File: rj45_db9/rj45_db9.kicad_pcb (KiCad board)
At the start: 2 copper layers, 30 x 32 mm, 2 parts, among them J1 RJ45_LED, J2 DB9_Female

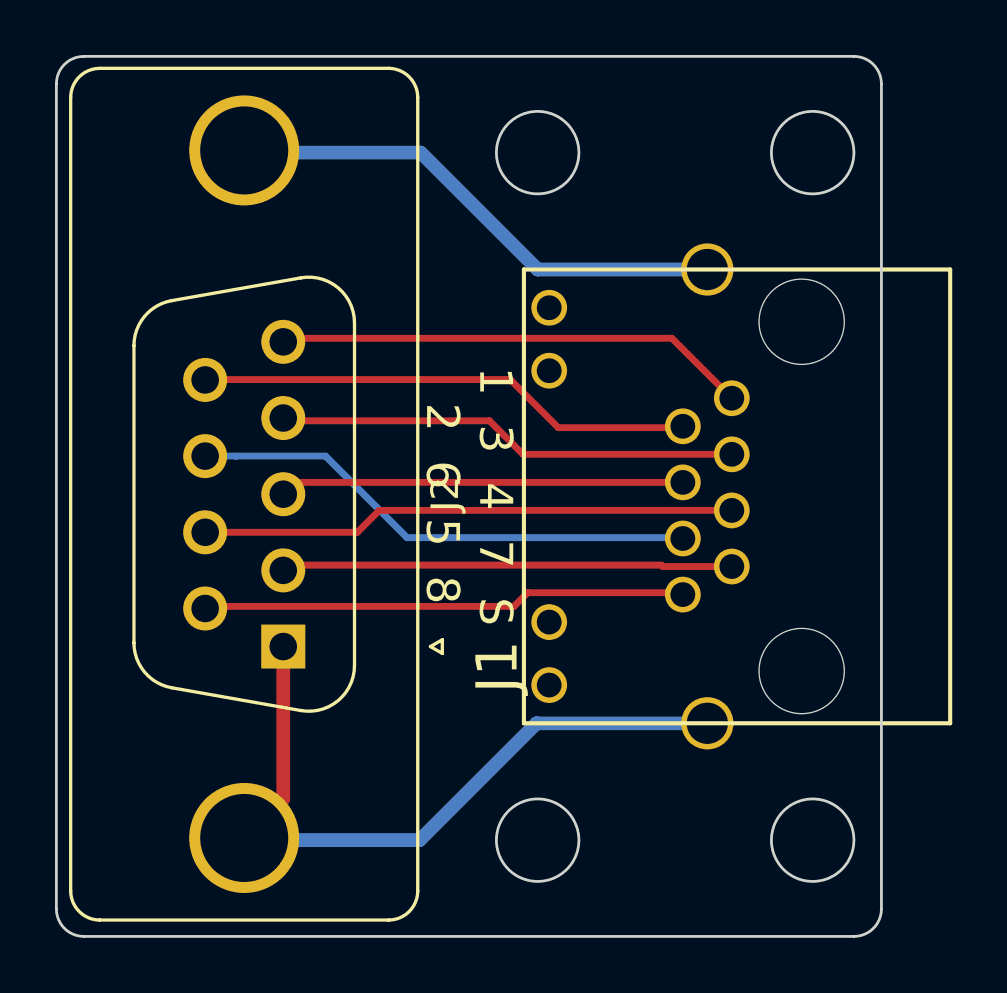
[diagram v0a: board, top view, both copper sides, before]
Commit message: hw
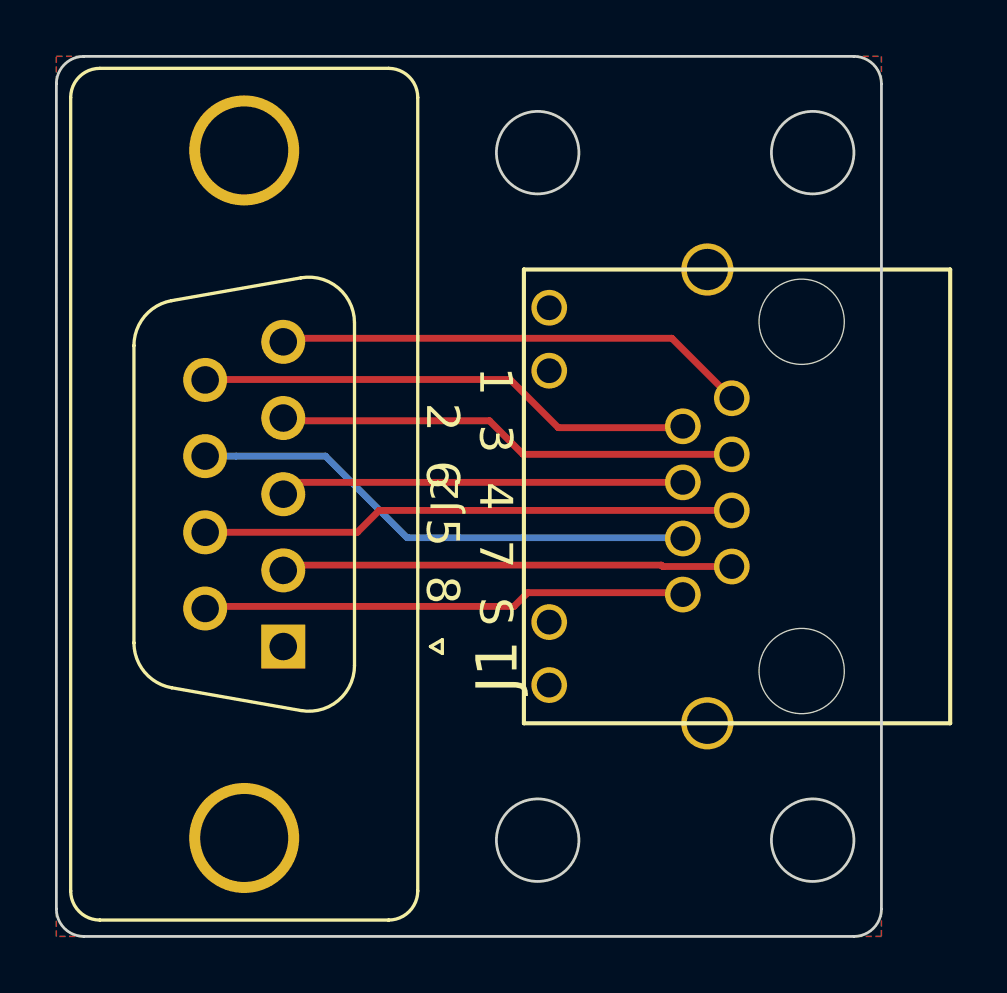
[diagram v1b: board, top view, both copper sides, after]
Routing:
- net Net-(J1-Pad13): track 44.6 -> 0.00 mm
- added copper zone on B.Cu, net Net-(J1-Pad13)
- added copper zone on F.Cu, net Net-(J1-Pad13)
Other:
- net class Default: via_dia 0.8 -> 0.6; via_drill 0.4 -> 0.3
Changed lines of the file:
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@@
     (thickness 1.6)
     (drawings 13)
-    (tracks 39)
+    (tracks 31)
     (zones 0)
     (modules 2)
@@
     (last_trace_width 0.25)
     (trace_clearance 0.2)
-    (zone_clearance 0.508)
+    (zone_clearance 0.2)
     (zone_45_only no)
     (trace_min 0.2)
-    (via_size 0.8)
-    (via_drill 0.4)
+    (via_size 0.6)
+    (via_drill 0.3)
     (via_min_size 0.4)
     (via_min_drill 0.3)
@@
     (clearance 0.2)
     (trace_width 0.25)
-    (via_dia 0.8)
-    (via_drill 0.4)
+    (via_dia 0.6)
+    (via_drill 0.3)
     (uvia_dia 0.3)
     (uvia_drill 0.1)
     (add_net "Net-(J1-Pad1)")
-    (add_net "Net-(J1-Pad10)")
-    (add_net "Net-(J1-Pad11)")
-    (add_net "Net-(J1-Pad12)")
     (add_net "Net-(J1-Pad13)")
     (add_net "Net-(J1-Pad2)")
@@
     (add_net "Net-(J1-Pad7)")
     (add_net "Net-(J1-Pad8)")
-    (add_net "Net-(J1-Pad9)")
   )
   (module stmbl:DSUB-9_Female_Vertical_Pitch2.77x2.84mm_MountingHoles (layer F.Cu)
@@
   (gr_line (start 143.5 116) (end 171.5 116) (layer Edge.Cuts) (width 0.1))
   (gr_line (start 142.5 85) (end 142.5 115) (layer Edge.Cuts) (width 0.1))
-  (segment (start 160 91.75) (end 166.17 91.75) (width 0.5) (layer B.Cu) (net 1))
-  (segment (start 155.75 87.5) (end 160 91.75) (width 0.5) (layer B.Cu) (net 1))
-  (segment (start 149.42 87.5) (end 155.75 87.5) (width 0.5) (layer B.Cu) (net 1))
-  (segment (start 155.71 112.5) (end 159.96 108.25) (width 0.5) (layer B.Cu) (net 1))
-  (segment (start 159.96 108.25) (end 166.17 108.25) (width 0.5) (layer B.Cu) (net 1))
-  (segment (start 149.42 112.5) (end 155.71 112.5) (width 0.5) (layer B.Cu) (net 1))
-  (segment (start 150.75 111) (end 150.75 105.46) (width 0.5) (layer F.Cu) (net 1))
-  (segment (start 149.33 112.42) (end 150.75 111) (width 0.5) (layer F.Cu) (net 1))
   (segment (start 164.88 94.25) (end 167.06 96.43) (width 0.25) (layer F.Cu) (net 2))
   (segment (start 150.75 94.38) (end 150.88 94.25) (width 0.25) (layer F.Cu) (net 2))
@@
   (segment (start 159.14 104) (end 159.64 103.5) (width 0.25) (layer F.Cu) (net 9))
   (segment (start 159.64 103.5) (end 165.21 103.5) (width 0.25) (layer F.Cu) (net 9))
+  (zone (net 1) (net_name "Net-(J1-Pad13)") (layer F.Cu) (hatch edge 0.508)
+    (connect_pads (clearance 0.2))
+    (min_thickness 0.2)
+    (fill yes (arc_segments 32) (thermal_gap 0.2) (thermal_bridge_width 0.25))
+    (polygon
+      (pts
+        (xy 142.5 84) (xy 172.5 84) (xy 172.5 116) (xy 142.5 116)
+      )
+    )
+  )
+  (zone (net 1) (net_name "Net-(J1-Pad13)") (layer B.Cu) (hatch edge 0.508)
+    (connect_pads (clearance 0.2))
+    (min_thickness 0.2)
+    (fill yes (arc_segments 32) (thermal_gap 0.2) (thermal_bridge_width 0.25))
+    (polygon
+      (pts
+        (xy 142.5 84) (xy 172.5 84) (xy 172.5 116) (xy 142.5 116)
+      )
+    )
+  )
+  (zone (net 0) (net_name "") (layers F&B.Cu) (hatch edge 0.508)
+    (connect_pads (clearance 0.2))
+    (min_thickness 0.2)
+    (keepout (tracks not_allowed) (vias not_allowed) (copperpour not_allowed))
+    (fill (arc_segments 32) (thermal_gap 0.2) (thermal_bridge_width 0.25))
+    (polygon
+      (pts
+        (xy 160 108.75) (xy 162 108.75) (xy 163.75 110.5) (xy 163.75 116) (xy 156.25 116)
+        (xy 156.25 110.5) (xy 158 108.75)
+      )
+    )
+  )
+  (zone (net 0) (net_name "") (layers F&B.Cu) (hatch edge 0.508)
+    (connect_pads (clearance 0.2))
+    (min_thickness 0.2)
+    (keepout (tracks not_allowed) (vias not_allowed) (copperpour not_allowed))
+    (fill (arc_segments 32) (thermal_gap 0.2) (thermal_bridge_width 0.25))
+    (polygon
+      (pts
+        (xy 169.978671 108.75) (xy 172.478671 108.75) (xy 173.728671 110) (xy 173.728671 116) (xy 166.228671 116)
+        (xy 166.25 110.5) (xy 168 108.75)
+      )
+    )
+  )
+  (zone (net 0) (net_name "") (layers F&B.Cu) (hatch edge 0.508)
+    (connect_pads (clearance 0.2))
+    (min_thickness 0.2)
+    (keepout (tracks not_allowed) (vias not_allowed) (copperpour not_allowed))
+    (fill (arc_segments 32) (thermal_gap 0.2) (thermal_bridge_width 0.25))
+    (polygon
+      (pts
+        (xy 170 91.25) (xy 168 91.25) (xy 166.25 89.5) (xy 166.25 84) (xy 173.75 84)
+        (xy 173.75 90) (xy 172.5 91.25)
+      )
+    )
+  )
+  (zone (net 0) (net_name "") (layers F&B.Cu) (hatch edge 0.508)
+    (connect_pads (clearance 0.2))
+    (min_thickness 0.2)
+    (keepout (tracks not_allowed) (vias not_allowed) (copperpour not_allowed))
+    (fill (arc_segments 32) (thermal_gap 0.2) (thermal_bridge_width 0.25))
+    (polygon
+      (pts
+        (xy 160 91.25) (xy 158 91.25) (xy 156.25 89.5) (xy 156.25 84) (xy 163.75 84)
+        (xy 163.75 89.5) (xy 162 91.25)
+      )
+    )
+  )
 )
